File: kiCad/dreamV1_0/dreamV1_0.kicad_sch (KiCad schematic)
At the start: 35 parts, among them IC1 TGS2611-C00, J1 GPIO, J11 10132328-10011LF, J2 Qwiic_Vertical, J3 679305124022, J4 Qwiic_Vertical, J5 M20-7830542, J6 Qwiic_Vertical, J7 5013310607, J8 Qwiic_Vertical, J9 Qwiic_Vertical, Q1 BSS138, U1 AP2112K-3.3, U2 BME280, U3 INA219BxDCN

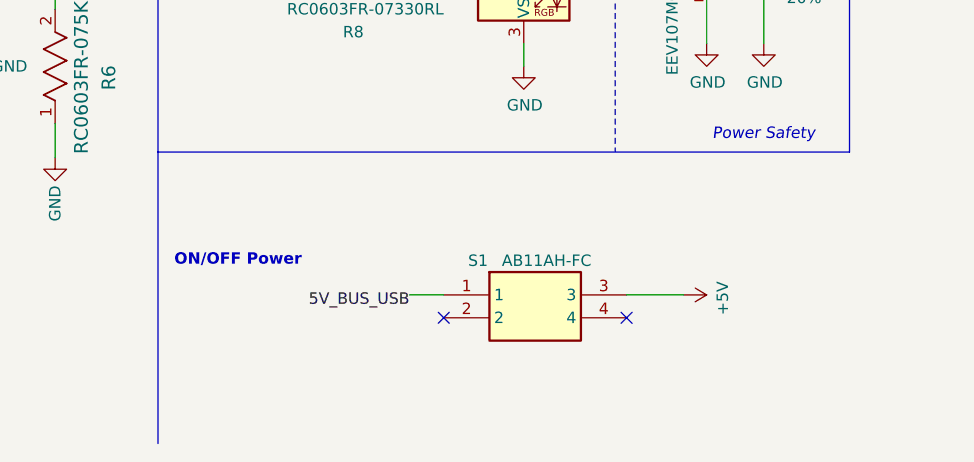
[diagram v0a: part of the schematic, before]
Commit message: Add files via upload
Type C moved to be above the GPIO, new switch, subtle mounting hole, and border changes.
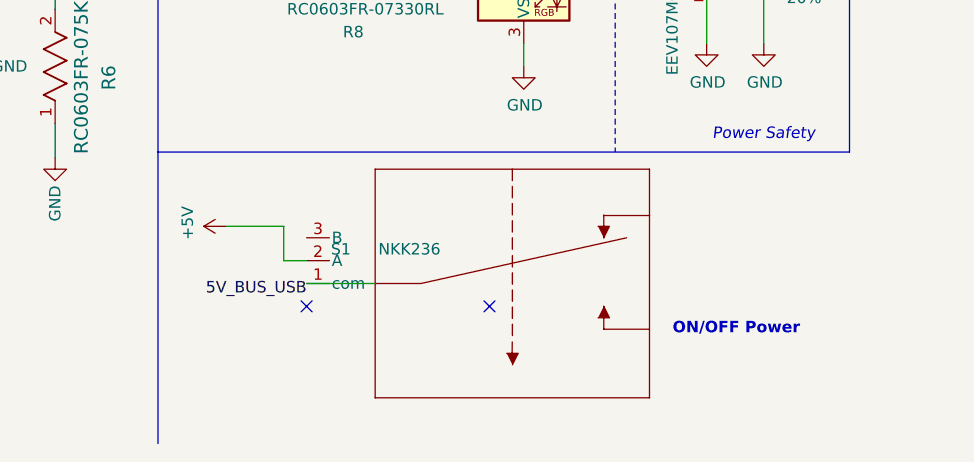
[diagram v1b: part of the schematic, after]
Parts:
- IC1: footprint TGS2611C00 -> footprints1:TGS2611-C00_FGS
- R7: footprint RC0603N_YAG-L -> Resistor_SMD:R_0603_1608Metric
- S1: value AB11AH-FC -> NKK236; footprint downloaded:AB11AHFC -> SWITCH_NK236_APM; symbol AB11AH-FC:AB11AH-FC -> 2025-12-31_23-00-22:NK236
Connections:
- net +5V: now also S1.2 (A); no longer S1.3
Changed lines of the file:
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@@
 	(text "ON/OFF Power"
 		(exclude_from_sim no)
-		(at 109.22 177.8 0)
+		(at 164.592 185.42 0)
 		(effects
 			(font
@@
 	)
 	(no_connect
-		(at 152.4 184.15)
+		(at 137.16 182.88)
 	)
 	(no_connect
@@
 	)
 	(no_connect
-		(at 132.08 184.15)
+		(at 116.84 182.88)
 	)
 	(no_connect
@@
 	(wire
 		(pts
+			(xy 114.3 173.99) (xy 114.3 177.8)
+		)
+		(stroke
+			(width 0)
+			(type default)
+		)
+	)
+	(wire
+		(pts
 			(xy 30.48 171.45) (xy 30.48 173.99)
 		)
@@
 	(wire
 		(pts
-			(xy 128.27 181.61) (xy 132.08 181.61)
+			(xy 124.46 180.34) (xy 116.84 180.34)
 		)
 		(stroke
@@
 	(wire
 		(pts
-			(xy 152.4 181.61) (xy 158.75 181.61)
-		)
-		(stroke
-			(width 0)
-			(type default)
-		)
-	)
-	(wire
-		(pts
 			(xy 264.16 134.62) (xy 267.97 134.62)
 		)
@@
 	(wire
 		(pts
+			(xy 114.3 177.8) (xy 116.84 177.8)
+		)
+		(stroke
+			(width 0)
+			(type default)
+		)
+	)
+	(wire
+		(pts
 			(xy 128.27 107.95) (xy 128.27 114.3)
 		)
@@
 	(wire
 		(pts
+			(xy 114.3 173.99) (xy 107.95 173.99)
+		)
+		(stroke
+			(width 0)
+			(type default)
+		)
+	)
+	(wire
+		(pts
 			(xy 35.56 148.59) (xy 32.385 148.59)
 		)
@@
 	)
 	(label "5V_BUS_USB"
-		(at 128.27 181.61 180)
+		(at 116.84 180.34 180)
 		(effects
 			(font
@@
 			)
 		)
-		(property "Footprint" "RC0603N_YAG-L"
+		(property "Footprint" "Resistor_SMD:R_0603_1608Metric"
 			(at 21.59 143.51 0)
 			(effects
@@
 	(symbol
 		(lib_id "power:+5V")
-		(at 158.75 181.61 270)
+		(at 107.95 173.99 90)
 		(unit 1)
 		(exclude_from_sim no)
@@
 		(dnp no)
 		(property "Reference" "#PWR058"
-			(at 154.94 181.61 0)
+			(at 111.76 173.99 0)
 			(effects
 				(font
@@
 		)
 		(property "Value" "+5V"
-			(at 163.0744 181.9783 0)
+			(at 103.6256 173.6217 0)
 			(effects
 				(font
@@
 		)
 		(property "Footprint" ""
-			(at 158.75 181.61 0)
+			(at 107.95 173.99 0)
 			(effects
 				(font
@@
 		)
 		(property "Datasheet" ""
-			(at 158.75 181.61 0)
+			(at 107.95 173.99 0)
 			(effects
 				(font
@@
 		)
 		(property "Description" "Power symbol creates a global label with name \"+5V\""
-			(at 158.75 181.61 0)
+			(at 107.95 173.99 0)
 			(effects
 				(font
@@
 	)
 	(symbol
-		(lib_id "AB11AH-FC:AB11AH-FC")
-		(at 132.08 181.61 0)
+		(lib_id "2025-12-31_23-00-22:NK236")
+		(at 116.84 180.34 0)
 		(unit 1)
 		(exclude_from_sim no)
@@
 		(dnp no)
 		(property "Reference" "S1"
-			(at 135.89 177.8 0)
+			(at 120.65 176.53 0)
 			(effects
 				(font
@@
 			)
 		)
-		(property "Value" "AB11AH-FC"
-			(at 143.51 177.8 0)
+		(property "Value" "NKK236"
+			(at 128.27 176.53 0)
 			(effects
 				(font
@@
 			)
 		)
-		(property "Footprint" "downloaded:AB11AHFC"
-			(at 148.59 276.53 0)
+		(property "Footprint" "SWITCH_NK236_APM"
+			(at 116.84 180.34 0)
 			(effects
 				(font
 					(size 1.27 1.27)
+					(italic yes)
 				)
-				(justify left top)
 				(hide yes)
 			)
 		)
-		(property "Datasheet" "https://static6.arrow.com/aropdfconversion/5ffd941f0a79b79b64ad9b37dc4e3b7206520647/pushbutton_ab.pdf"
-			(at 148.59 376.53 0)
+		(property "Datasheet" "NK236"
+			(at 116.84 180.34 0)
 			(effects
 				(font
 					(size 1.27 1.27)
+					(italic yes)
 				)
-				(justify left top)
 				(hide yes)
 			)
 		)
 		(property "Description" "Pushbutton Switches OFF-(ON) .201 RD CAP RIGHT ANGL PC .4VA Process Sealed Subminiature Pushbuttons"
-			(at 132.08 181.61 0)
+			(at 116.84 180.34 0)
 			(effects
 				(font
@@
 		)
 		(property "Height" "6.18"
-			(at 148.59 576.53 0)
+			(at 133.35 575.26 0)
 			(effects
 				(font
@@
 		)
 		(property "Mouser Part Number" "633-AB11AH-FC"
-			(at 148.59 676.53 0)
+			(at 133.35 675.26 0)
 			(effects
 				(font
@@
 		)
 		(property "Mouser Price/Stock" "https://www.mouser.co.uk/ProductDetail/NKK-Switches/AB11AH-FC?qs=E3XkhTW0K2FjNZbXLHs%252BZw%3D%3D"
-			(at 148.59 776.53 0)
+			(at 133.35 775.26 0)
 			(effects
 				(font
@@
 		)
 		(property "Manufacturer_Name" "NKK Switches"
-			(at 148.59 876.53 0)
+			(at 133.35 875.26 0)
 			(effects
 				(font
@@
 		)
 		(property "Manufacturer_Part_Number" "AB11AH-FC"
-			(at 148.59 976.53 0)
+			(at 133.35 975.26 0)
 			(effects
 				(font
@@
 		)
 		(property "Vendor" "https://www.digikey.com/en/products/detail/nkk-switches/AB11AH-FC/1055910?s=N4IgTCBcDaIIICECMS4AkC0AxAwiAugL5A"
-			(at 132.08 181.61 0)
+			(at 116.84 180.34 0)
 			(effects
 				(font
@@
 			)
 		)
-		(pin "3"
-		)
-		(pin "4"
-		)
 		(pin "1"
 		)
+		(pin "3"
+		)
 		(pin "2"
 		)
@@
 			)
 		)
-		(property "Footprint" "TGS2611C00"
+		(property "Footprint" "footprints1:TGS2611-C00_FGS"
 			(at 275.59 202.87 0)
 			(effects

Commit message: reverted file structure to contain both v1 and v2
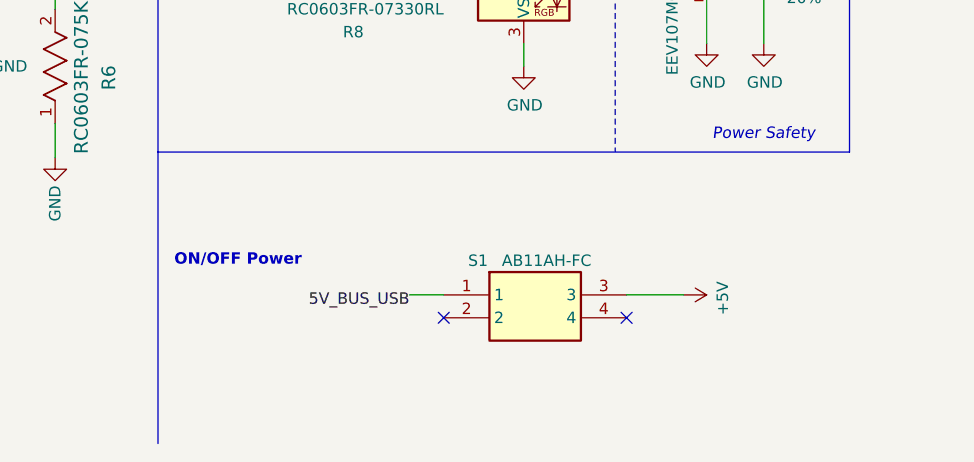
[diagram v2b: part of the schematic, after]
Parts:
- IC1: footprint footprints1:TGS2611-C00_FGS -> TGS2611C00
- R7: footprint Resistor_SMD:R_0603_1608Metric -> RC0603N_YAG-L
- S1: value NKK236 -> AB11AH-FC; footprint SWITCH_NK236_APM -> downloaded:AB11AHFC; symbol 2025-12-31_23-00-22:NK236 -> AB11AH-FC:AB11AH-FC
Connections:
- net +5V: now also S1.3; no longer S1.2 (A)
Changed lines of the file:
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@@
 	(text "ON/OFF Power"
 		(exclude_from_sim no)
-		(at 164.592 185.42 0)
+		(at 109.22 177.8 0)
 		(effects
 			(font
@@
 	)
 	(no_connect
-		(at 137.16 182.88)
+		(at 152.4 184.15)
 	)
 	(no_connect
@@
 	)
 	(no_connect
-		(at 116.84 182.88)
+		(at 132.08 184.15)
 	)
 	(no_connect
@@
 	(wire
 		(pts
-			(xy 114.3 173.99) (xy 114.3 177.8)
-		)
-		(stroke
-			(width 0)
-			(type default)
-		)
-	)
-	(wire
-		(pts
 			(xy 30.48 171.45) (xy 30.48 173.99)
 		)
@@
 	(wire
 		(pts
-			(xy 124.46 180.34) (xy 116.84 180.34)
+			(xy 128.27 181.61) (xy 132.08 181.61)
 		)
 		(stroke
@@
 	(wire
 		(pts
+			(xy 152.4 181.61) (xy 158.75 181.61)
+		)
+		(stroke
+			(width 0)
+			(type default)
+		)
+	)
+	(wire
+		(pts
 			(xy 264.16 134.62) (xy 267.97 134.62)
 		)
@@
 	(wire
 		(pts
-			(xy 114.3 177.8) (xy 116.84 177.8)
-		)
-		(stroke
-			(width 0)
-			(type default)
-		)
-	)
-	(wire
-		(pts
 			(xy 128.27 107.95) (xy 128.27 114.3)
 		)
@@
 	(wire
 		(pts
-			(xy 114.3 173.99) (xy 107.95 173.99)
-		)
-		(stroke
-			(width 0)
-			(type default)
-		)
-	)
-	(wire
-		(pts
 			(xy 35.56 148.59) (xy 32.385 148.59)
 		)
@@
 	)
 	(label "5V_BUS_USB"
-		(at 116.84 180.34 180)
+		(at 128.27 181.61 180)
 		(effects
 			(font
@@
 			)
 		)
-		(property "Footprint" "Resistor_SMD:R_0603_1608Metric"
+		(property "Footprint" "RC0603N_YAG-L"
 			(at 21.59 143.51 0)
 			(effects
@@
 	(symbol
 		(lib_id "power:+5V")
-		(at 107.95 173.99 90)
+		(at 158.75 181.61 270)
 		(unit 1)
 		(exclude_from_sim no)
@@
 		(dnp no)
 		(property "Reference" "#PWR058"
-			(at 111.76 173.99 0)
+			(at 154.94 181.61 0)
 			(effects
 				(font
@@
 		)
 		(property "Value" "+5V"
-			(at 103.6256 173.6217 0)
+			(at 163.0744 181.9783 0)
 			(effects
 				(font
@@
 		)
 		(property "Footprint" ""
-			(at 107.95 173.99 0)
+			(at 158.75 181.61 0)
 			(effects
 				(font
@@
 		)
 		(property "Datasheet" ""
-			(at 107.95 173.99 0)
+			(at 158.75 181.61 0)
 			(effects
 				(font
@@
 		)
 		(property "Description" "Power symbol creates a global label with name \"+5V\""
-			(at 107.95 173.99 0)
+			(at 158.75 181.61 0)
 			(effects
 				(font
@@
 	)
 	(symbol
-		(lib_id "2025-12-31_23-00-22:NK236")
-		(at 116.84 180.34 0)
+		(lib_id "AB11AH-FC:AB11AH-FC")
+		(at 132.08 181.61 0)
 		(unit 1)
 		(exclude_from_sim no)
@@
 		(dnp no)
 		(property "Reference" "S1"
-			(at 120.65 176.53 0)
+			(at 135.89 177.8 0)
 			(effects
 				(font
@@
 			)
 		)
-		(property "Value" "NKK236"
-			(at 128.27 176.53 0)
+		(property "Value" "AB11AH-FC"
+			(at 143.51 177.8 0)
 			(effects
 				(font
@@
 			)
 		)
-		(property "Footprint" "SWITCH_NK236_APM"
-			(at 116.84 180.34 0)
+		(property "Footprint" "downloaded:AB11AHFC"
+			(at 148.59 276.53 0)
 			(effects
 				(font
 					(size 1.27 1.27)
-					(italic yes)
 				)
+				(justify left top)
 				(hide yes)
 			)
 		)
-		(property "Datasheet" "NK236"
-			(at 116.84 180.34 0)
+		(property "Datasheet" "https://static6.arrow.com/aropdfconversion/5ffd941f0a79b79b64ad9b37dc4e3b7206520647/pushbutton_ab.pdf"
+			(at 148.59 376.53 0)
 			(effects
 				(font
 					(size 1.27 1.27)
-					(italic yes)
 				)
+				(justify left top)
 				(hide yes)
 			)
 		)
 		(property "Description" "Pushbutton Switches OFF-(ON) .201 RD CAP RIGHT ANGL PC .4VA Process Sealed Subminiature Pushbuttons"
-			(at 116.84 180.34 0)
+			(at 132.08 181.61 0)
 			(effects
 				(font
@@
 		)
 		(property "Height" "6.18"
-			(at 133.35 575.26 0)
+			(at 148.59 576.53 0)
 			(effects
 				(font
@@
 		)
 		(property "Mouser Part Number" "633-AB11AH-FC"
-			(at 133.35 675.26 0)
+			(at 148.59 676.53 0)
 			(effects
 				(font
@@
 		)
 		(property "Mouser Price/Stock" "https://www.mouser.co.uk/ProductDetail/NKK-Switches/AB11AH-FC?qs=E3XkhTW0K2FjNZbXLHs%252BZw%3D%3D"
-			(at 133.35 775.26 0)
+			(at 148.59 776.53 0)
 			(effects
 				(font
@@
 		)
 		(property "Manufacturer_Name" "NKK Switches"
-			(at 133.35 875.26 0)
+			(at 148.59 876.53 0)
 			(effects
 				(font
@@
 		)
 		(property "Manufacturer_Part_Number" "AB11AH-FC"
-			(at 133.35 975.26 0)
+			(at 148.59 976.53 0)
 			(effects
 				(font
@@
 		)
 		(property "Vendor" "https://www.digikey.com/en/products/detail/nkk-switches/AB11AH-FC/1055910?s=N4IgTCBcDaIIICECMS4AkC0AxAwiAugL5A"
-			(at 116.84 180.34 0)
+			(at 132.08 181.61 0)
 			(effects
 				(font
@@
 			)
 		)
-		(pin "1"
-		)
 		(pin "3"
 		)
+		(pin "4"
+		)
+		(pin "1"
+		)
 		(pin "2"
 		)
@@
 			)
 		)
-		(property "Footprint" "footprints1:TGS2611-C00_FGS"
+		(property "Footprint" "TGS2611C00"
 			(at 275.59 202.87 0)
 			(effects
